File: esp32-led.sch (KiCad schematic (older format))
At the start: 10 parts, among them J1 LED Connector, J2 USB4125-GF-A_REVA2, J3 LED Connector, U1 SN74AHCT125D, U2 ESP32_NODEMCU

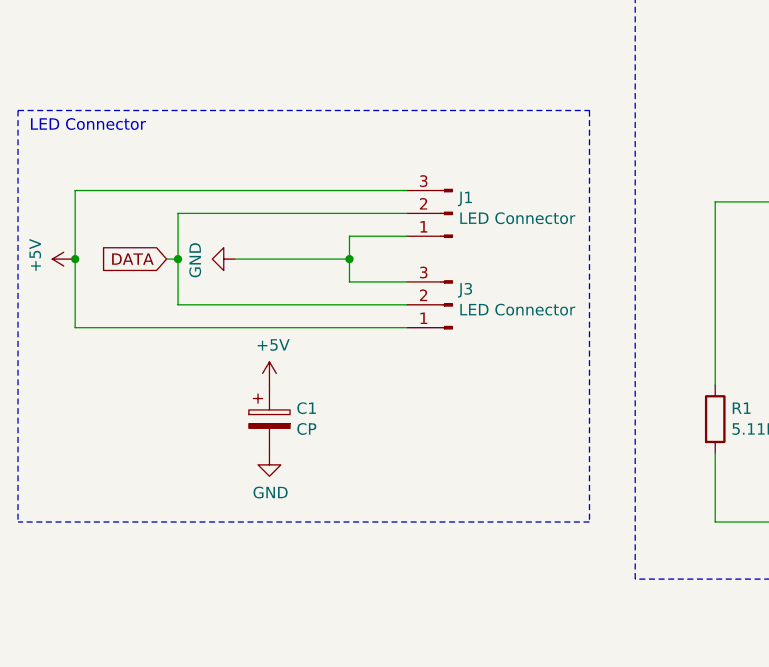
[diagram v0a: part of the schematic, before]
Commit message: Fixed issues, added gerber files
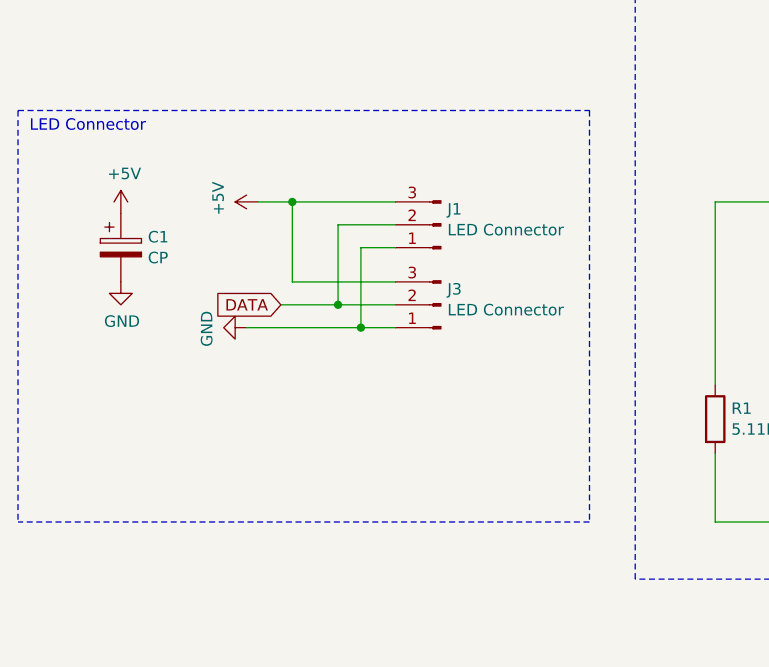
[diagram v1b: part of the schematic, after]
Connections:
- net +5V: now also J3.3 (Pin_3); no longer J3.1 (Pin_1)
- net GND: now also J3.1 (Pin_1); no longer J3.3 (Pin_3)
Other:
- moved on the sheet: C1, J1, J3
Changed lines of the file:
@@
 Wire Notes Line
 	3450 3600 950  3600
-Text GLabel 1600 2450 0    50   Input ~ 0
+Text GLabel 2100 2650 0    50   Input ~ 0
 DATA
 $Comp
 L Connector:Conn_01x03_Male J1
 U 1 1 62EB48AB
-P 2850 2250
-F 0 "J1" H 2822 2182 50  0000 R CNN
-F 1 "LED Connector" H 2822 2273 50  0000 R CNN
-F 2 "Connector_PinHeader_2.54mm:PinHeader_1x03_P2.54mm_Vertical" H 2850 2250 50  0001 C CNN
-F 3 "~" H 2850 2250 50  0001 C CNN
-	1    2850 2250
+P 2800 2300
+F 0 "J1" H 2772 2232 50  0000 R CNN
+F 1 "LED Connector" H 2772 2323 50  0000 R CNN
+F 2 "Connector_PinHeader_2.54mm:PinHeader_1x03_P2.54mm_Vertical" H 2800 2300 50  0001 C CNN
+F 3 "~" H 2800 2300 50  0001 C CNN
+	1    2800 2300
 	-1   0    0    1
 $EndComp
@@
 L Device:CP C1
 U 1 1 62EB16DE
-P 2050 3150
-F 0 "C1" H 2168 3196 50  0000 L CNN
-F 1 "CP" H 2168 3105 50  0000 L CNN
-F 2 "Capacitor_THT:CP_Radial_D10.0mm_P5.00mm" H 2088 3000 50  0001 C CNN
-F 3 "~" H 2050 3150 50  0001 C CNN
-	1    2050 3150
+P 1400 2400
+F 0 "C1" H 1518 2446 50  0000 L CNN
+F 1 "CP" H 1518 2355 50  0000 L CNN
+F 2 "Capacitor_THT:CP_Radial_D10.0mm_P5.00mm" H 1438 2250 50  0001 C CNN
+F 3 "~" H 1400 2400 50  0001 C CNN
+	1    1400 2400
 	1    0    0    -1
 $EndComp
@@
 L power:+5V #PWR01
 U 1 1 62EB0400
-P 1200 2450
-F 0 "#PWR01" H 1200 2300 50  0001 C CNN
-F 1 "+5V" H 1215 2623 50  0000 C CNN
-F 2 "" H 1200 2450 50  0001 C CNN
-F 3 "" H 1200 2450 50  0001 C CNN
-	1    1200 2450
+P 2000 2200
+F 0 "#PWR01" H 2000 2050 50  0001 C CNN
+F 1 "+5V" H 2015 2373 50  0000 C CNN
+F 2 "" H 2000 2200 50  0001 C CNN
+F 3 "" H 2000 2200 50  0001 C CNN
+	1    2000 2200
 	0    -1   -1   0
 $EndComp
@@
 L power:GND #PWR02
 U 1 1 62EAF6FE
-P 1900 2450
-F 0 "#PWR02" H 1900 2200 50  0001 C CNN
-F 1 "GND" H 1905 2277 50  0000 C CNN
-F 2 "" H 1900 2450 50  0001 C CNN
-F 3 "" H 1900 2450 50  0001 C CNN
-	1    1900 2450
+P 1950 2750
+F 0 "#PWR02" H 1950 2500 50  0001 C CNN
+F 1 "GND" H 1955 2577 50  0000 C CNN
+F 2 "" H 1950 2750 50  0001 C CNN
+F 3 "" H 1950 2750 50  0001 C CNN
+	1    1950 2750
 	0    1    1    0
 $EndComp
@@
 L Connector:Conn_01x03_Male J3
 U 1 1 62E912D3
-P 2850 2650
-F 0 "J3" H 2822 2582 50  0000 R CNN
-F 1 "LED Connector" H 2822 2673 50  0000 R CNN
-F 2 "Connector_PinHeader_2.54mm:PinHeader_1x03_P2.54mm_Vertical" H 2850 2650 50  0001 C CNN
-F 3 "~" H 2850 2650 50  0001 C CNN
-	1    2850 2650
+P 2800 2650
+F 0 "J3" H 2772 2582 50  0000 R CNN
+F 1 "LED Connector" H 2772 2673 50  0000 R CNN
+F 2 "Connector_PinHeader_2.54mm:PinHeader_1x03_P2.54mm_Vertical" H 2800 2650 50  0001 C CNN
+F 3 "~" H 2800 2650 50  0001 C CNN
+	1    2800 2650
 	-1   0    0    1
 $EndComp
-Wire Wire Line
-	1900 2450 2400 2450
-Wire Wire Line
-	2400 2450 2400 2350
-Wire Wire Line
-	2400 2350 2650 2350
-Wire Wire Line
-	2400 2450 2400 2550
-Wire Wire Line
-	2400 2550 2650 2550
-Connection ~ 2400 2450
-Wire Wire Line
-	1600 2450 1650 2450
-Wire Wire Line
-	1650 2450 1650 2250
-Wire Wire Line
-	1650 2250 2650 2250
-Wire Wire Line
-	1650 2450 1650 2650
-Wire Wire Line
-	1650 2650 2650 2650
-Connection ~ 1650 2450
-Wire Wire Line
-	1200 2450 1200 2150
-Wire Wire Line
-	1200 2450 1200 2750
-Wire Wire Line
-	1200 2750 2650 2750
-Connection ~ 1200 2450
-Wire Wire Line
-	1200 2150 2650 2150
 $Comp
 L power:+5V #PWR09
 U 1 1 62ED22FC
-P 2050 3000
-F 0 "#PWR09" H 2050 2850 50  0001 C CNN
-F 1 "+5V" H 2065 3173 50  0000 C CNN
-F 2 "" H 2050 3000 50  0001 C CNN
-F 3 "" H 2050 3000 50  0001 C CNN
-	1    2050 3000
+P 1400 2250
+F 0 "#PWR09" H 1400 2100 50  0001 C CNN
+F 1 "+5V" H 1415 2423 50  0000 C CNN
+F 2 "" H 1400 2250 50  0001 C CNN
+F 3 "" H 1400 2250 50  0001 C CNN
+	1    1400 2250
 	1    0    0    -1
 $EndComp
@@
 L power:GND #PWR010
 U 1 1 62ED32C8
-P 2050 3300
-F 0 "#PWR010" H 2050 3050 50  0001 C CNN
-F 1 "GND" H 2055 3127 50  0000 C CNN
-F 2 "" H 2050 3300 50  0001 C CNN
-F 3 "" H 2050 3300 50  0001 C CNN
-	1    2050 3300
+P 1400 2550
+F 0 "#PWR010" H 1400 2300 50  0001 C CNN
+F 1 "GND" H 1405 2377 50  0000 C CNN
+F 2 "" H 1400 2550 50  0001 C CNN
+F 3 "" H 1400 2550 50  0001 C CNN
+	1    1400 2550
 	1    0    0    -1
 $EndComp
@@
 Wire Notes Line
 	950  1800 950  3600
+Wire Wire Line
+	2600 2200 2150 2200
+Wire Wire Line
+	2150 2200 2150 2550
+Wire Wire Line
+	2150 2550 2600 2550
+Wire Wire Line
+	2150 2200 2000 2200
+Connection ~ 2150 2200
+Wire Wire Line
+	2600 2300 2350 2300
+Wire Wire Line
+	2350 2300 2350 2650
+Wire Wire Line
+	2350 2650 2600 2650
+Wire Wire Line
+	2100 2650 2350 2650
+Connection ~ 2350 2650
+Wire Wire Line
+	2600 2400 2450 2400
+Wire Wire Line
+	2450 2400 2450 2750
+Wire Wire Line
+	2450 2750 2600 2750
+Wire Wire Line
+	2450 2750 1950 2750
+Connection ~ 2450 2750
 $EndSCHEMATC
